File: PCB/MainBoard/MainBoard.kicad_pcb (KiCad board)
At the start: 2 copper layers, 100.1 x 78.2 mm, 54 parts, among them J1 Switch, J2 Prog Connector, J3 UART, J4 IR Connector, J5 R Motor, J6 L_Motor, J7 L_Motor_Backup, J8 R_Motor_Backup, J9 Backup connector bit, Q1 BSR802, Q2 BSR802, SW1 RESET_SW, U1 MCP1700-3302E/TO, U2 ATmega4808-A

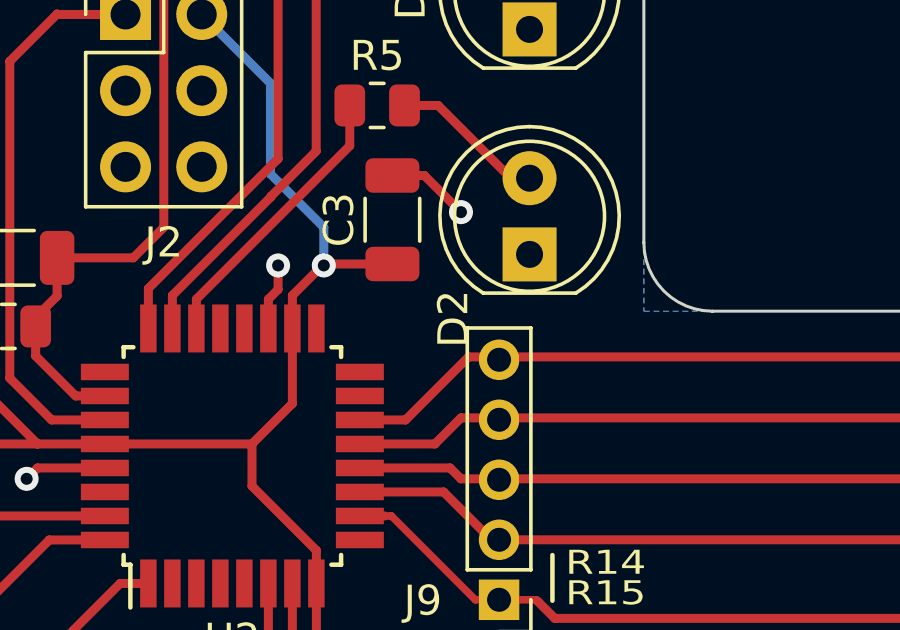
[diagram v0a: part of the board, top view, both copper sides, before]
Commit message: Cleaned up repo
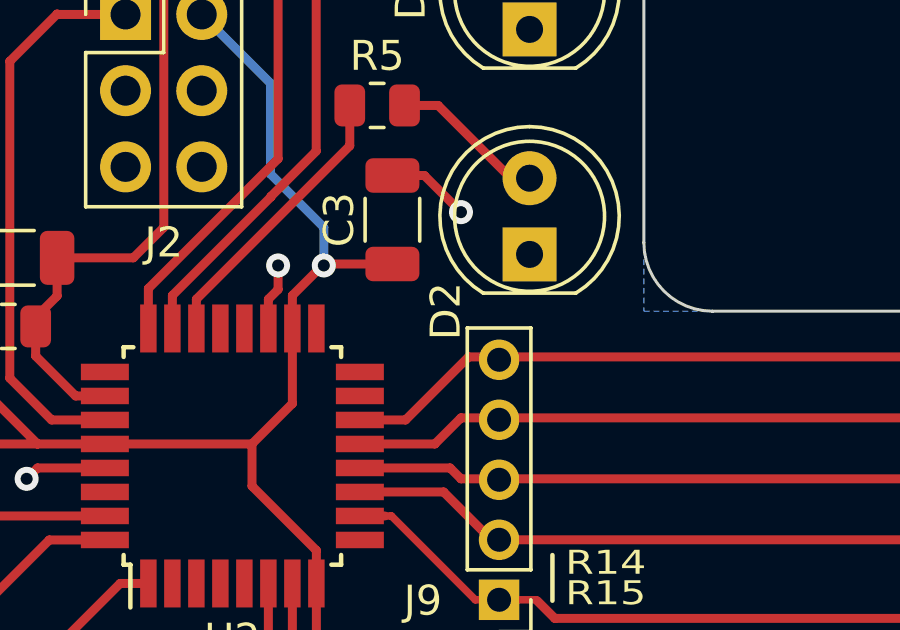
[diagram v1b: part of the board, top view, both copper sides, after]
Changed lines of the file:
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@@
     (property "ki_keywords" "LED diode")
     (attr through_hole)
-    (fp_text reference "D2" (at -2.147 -2.54 90) (layer "F.SilkS")
+    (fp_text reference "D2" (at -1.893 -2.794 90) (layer "F.SilkS")
         (effects (font (size 1 1) (thickness 0.15)))
     )
